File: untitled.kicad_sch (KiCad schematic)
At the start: 50 parts, among them J10 Conn_01x02, J11 Conn_01x02, J12 Conn_01x02, J13 Conn_01x02, J14 Conn_01x02, J15 Conn_01x02, J16 Conn_01x02, J17 Conn_01x02, J8 Conn_01x02, J9 Conn_01x02, Q11 Q_NMOS_GSD, Q12 Q_NMOS_GSD, Q13 Q_NMOS_GSD, Q14 Q_NMOS_GSD, Q15 Q_NMOS_GSD, Q16 Q_NMOS_GSD, Q17 Q_NMOS_GSD, Q18 Q_NMOS_GSD, Q19 Q_NMOS_GSD, Q20 Q_NMOS_GSD

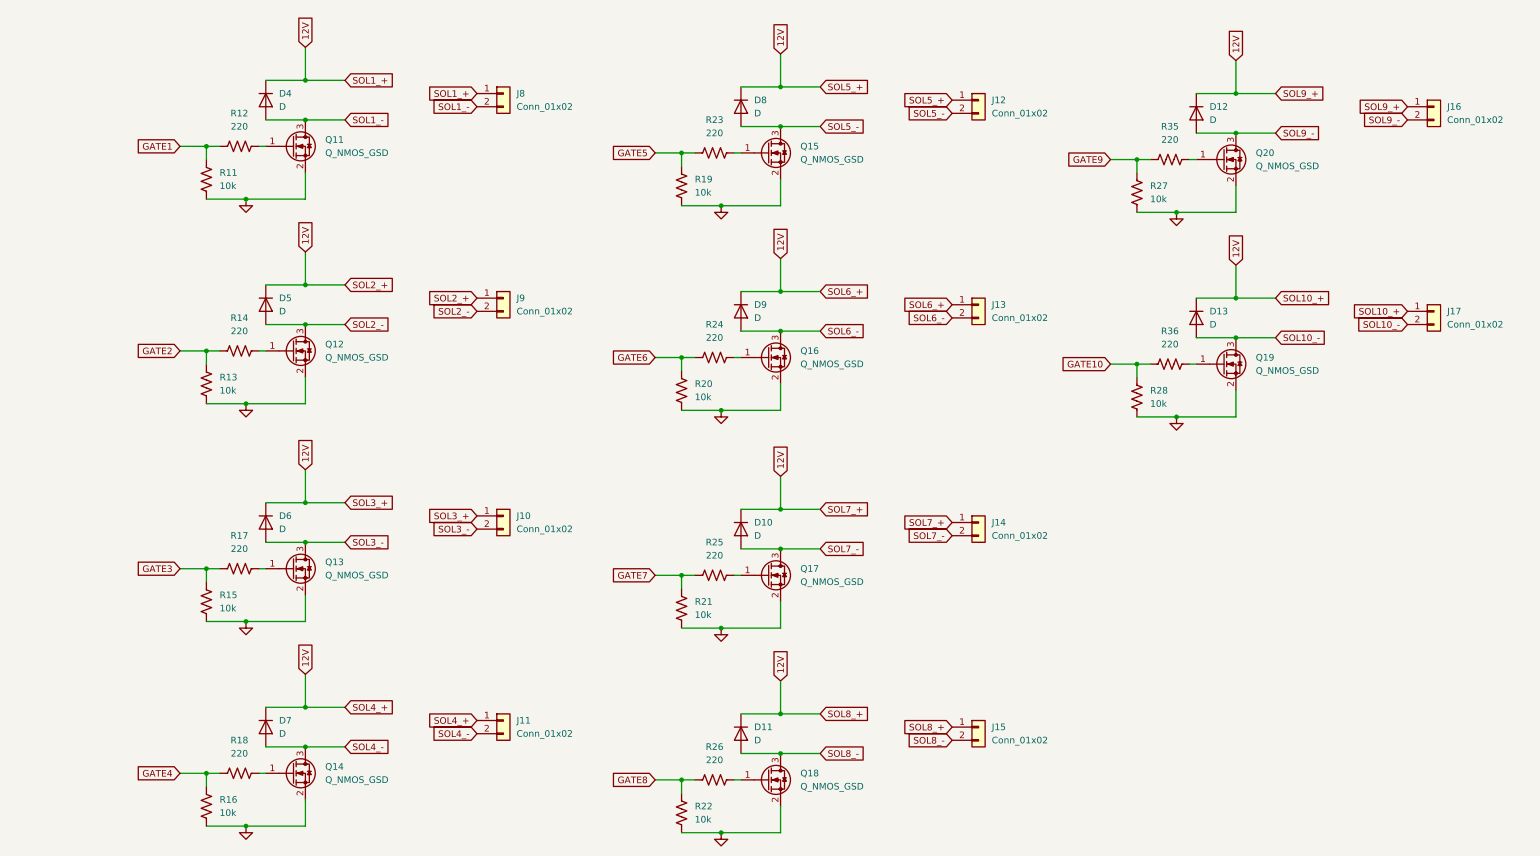
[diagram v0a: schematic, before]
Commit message: We are BACK
I am feeling myself. Lots of progress here.
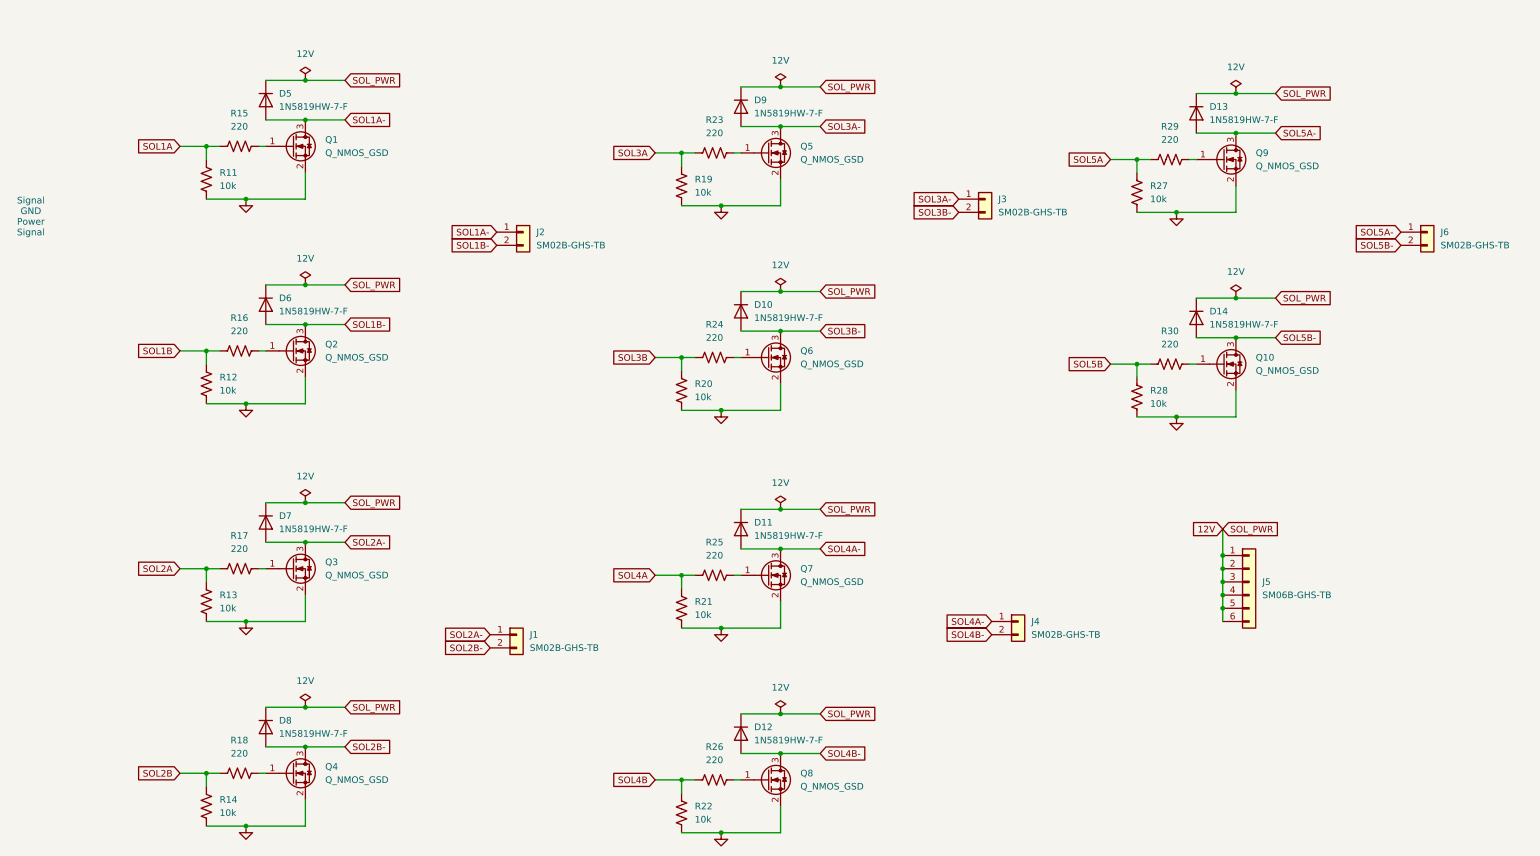
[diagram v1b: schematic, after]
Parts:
- removed J10, J11, J12, J13, J14, J15, J17, J8, J9: Conn_01x02, symbol Connector_Generic:Conn_01x02
- removed R13: 10k, symbol Device:R_US
- added J1, J2, J3, J4: SM02B-GHS-TB, x19_control_library:CONN_SM02B-GHS_JST, symbol Connector_Generic:Conn_01x02
- added J5: SM06B-GHS-TB, x19_control_library:CONN_SM06B-GHS-TB_JST, symbol Connector_Generic:Conn_01x06
- added R12: 10k, Resistor_SMD:R_0603_1608Metric_Pad0.98x0.95mm_HandSolder, symbol Device:R_US
- D10: renamed from D9; value D -> 1N5819HW-7-F; footprint (none) -> x19_control_library:1N5819HW-7-F_DIO
- D11: renamed from D10; value D -> 1N5819HW-7-F; footprint (none) -> x19_control_library:1N5819HW-7-F_DIO
- D12: renamed from D11; value D -> 1N5819HW-7-F; footprint (none) -> x19_control_library:1N5819HW-7-F_DIO
- D13: renamed from D12; value D -> 1N5819HW-7-F; footprint (none) -> x19_control_library:1N5819HW-7-F_DIO
- D14: renamed from D13; value D -> 1N5819HW-7-F; footprint (none) -> x19_control_library:1N5819HW-7-F_DIO
- D5: renamed from D4; value D -> 1N5819HW-7-F; footprint (none) -> x19_control_library:1N5819HW-7-F_DIO
- D6: renamed from D5; value D -> 1N5819HW-7-F; footprint (none) -> x19_control_library:1N5819HW-7-F_DIO
- D7: renamed from D6; value D -> 1N5819HW-7-F; footprint (none) -> x19_control_library:1N5819HW-7-F_DIO
- D8: renamed from D7; value D -> 1N5819HW-7-F; footprint (none) -> x19_control_library:1N5819HW-7-F_DIO
- D9: renamed from D8; value D -> 1N5819HW-7-F; footprint (none) -> x19_control_library:1N5819HW-7-F_DIO
- J6: renamed from J16; value Conn_01x02 -> SM02B-GHS-TB; footprint (none) -> x19_control_library:CONN_SM02B-GHS_JST
- Q1: renamed from Q11; footprint (none) -> x19_control_library:SOT-23-3L_AOS
- Q10: renamed from Q19; footprint (none) -> x19_control_library:SOT-23-3L_AOS
- Q2: renamed from Q12; footprint (none) -> x19_control_library:SOT-23-3L_AOS
- Q3: renamed from Q13; footprint (none) -> x19_control_library:SOT-23-3L_AOS
- Q4: renamed from Q14; footprint (none) -> x19_control_library:SOT-23-3L_AOS
- Q5: renamed from Q15; footprint (none) -> x19_control_library:SOT-23-3L_AOS
- Q6: renamed from Q16; footprint (none) -> x19_control_library:SOT-23-3L_AOS
- Q7: renamed from Q17; footprint (none) -> x19_control_library:SOT-23-3L_AOS
- Q8: renamed from Q18; footprint (none) -> x19_control_library:SOT-23-3L_AOS
- Q9: renamed from Q20; footprint (none) -> x19_control_library:SOT-23-3L_AOS
- R11, R17, R18, R19, R20, R21, R22, R23, R24, R25, R26, R27, R28: footprint (none) -> Resistor_SMD:R_0603_1608Metric_Pad0.98x0.95mm_HandSolder
- R13: renamed from R15; footprint (none) -> Resistor_SMD:R_0603_1608Metric_Pad0.98x0.95mm_HandSolder
- R14: renamed from R16; footprint (none) -> Resistor_SMD:R_0603_1608Metric_Pad0.98x0.95mm_HandSolder
- R15: renamed from R12; footprint (none) -> Resistor_SMD:R_0603_1608Metric_Pad0.98x0.95mm_HandSolder
- R16: renamed from R14; footprint (none) -> Resistor_SMD:R_0603_1608Metric_Pad0.98x0.95mm_HandSolder
- R29: renamed from R35; footprint (none) -> Resistor_SMD:R_0603_1608Metric_Pad0.98x0.95mm_HandSolder
- R30: renamed from R36; footprint (none) -> Resistor_SMD:R_0603_1608Metric_Pad0.98x0.95mm_HandSolder
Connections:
- net 12V: now also J5.1 (Pin_1), J5.2 (Pin_2), J5.3 (Pin_3), J5.4 (Pin_4), J5.5 (Pin_5), J5.6 (Pin_6); no longer J6.1 (Pin_1)
- net GND: now also R12.2
- net GATE1 renamed SOL1A
- net GATE10 renamed SOL5B
- net GATE2 renamed SOL1B
- net SOL1B: now also R12.1
- net GATE3 renamed SOL2A
- net GATE4 renamed SOL2B
- net GATE5 renamed SOL3A
- net GATE6 renamed SOL3B
- net GATE7 renamed SOL4A
- net GATE8 renamed SOL4B
- net GATE9 renamed SOL5A
- net SOL10_- renamed SOL5B-
- net SOL5B-: now also J6.2 (Pin_2)
- net SOL1_- renamed SOL1A-
- net SOL1A-: now also J2.1 (Pin_1)
- net SOL2_- renamed SOL1B-
- net SOL1B-: now also J2.2 (Pin_2)
- net SOL3_- renamed SOL2A-
- net SOL2A-: now also J1.1 (Pin_1)
- net SOL4_- renamed SOL2B-
- net SOL2B-: now also J1.2 (Pin_2)
- net SOL5_- renamed SOL3A-
- net SOL3A-: now also J3.1 (Pin_1)
- net SOL6_- renamed SOL3B-
- net SOL3B-: now also J3.2 (Pin_2)
- net SOL7_- renamed SOL4A-
- net SOL4A-: now also J4.1 (Pin_1)
- net SOL8_- renamed SOL4B-
- net SOL4B-: now also J4.2 (Pin_2)
- net SOL9_- renamed SOL5A-
- net SOL5A-: now also J6.1 (Pin_1); no longer J6.2 (Pin_2)
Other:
- note added: "Signal GND Power Signal"
- moved on the sheet: J6
